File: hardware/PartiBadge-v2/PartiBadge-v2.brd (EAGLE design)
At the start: 119.8 x 118.6 mm, 32 parts, among them J1 I2C, J2 Supply

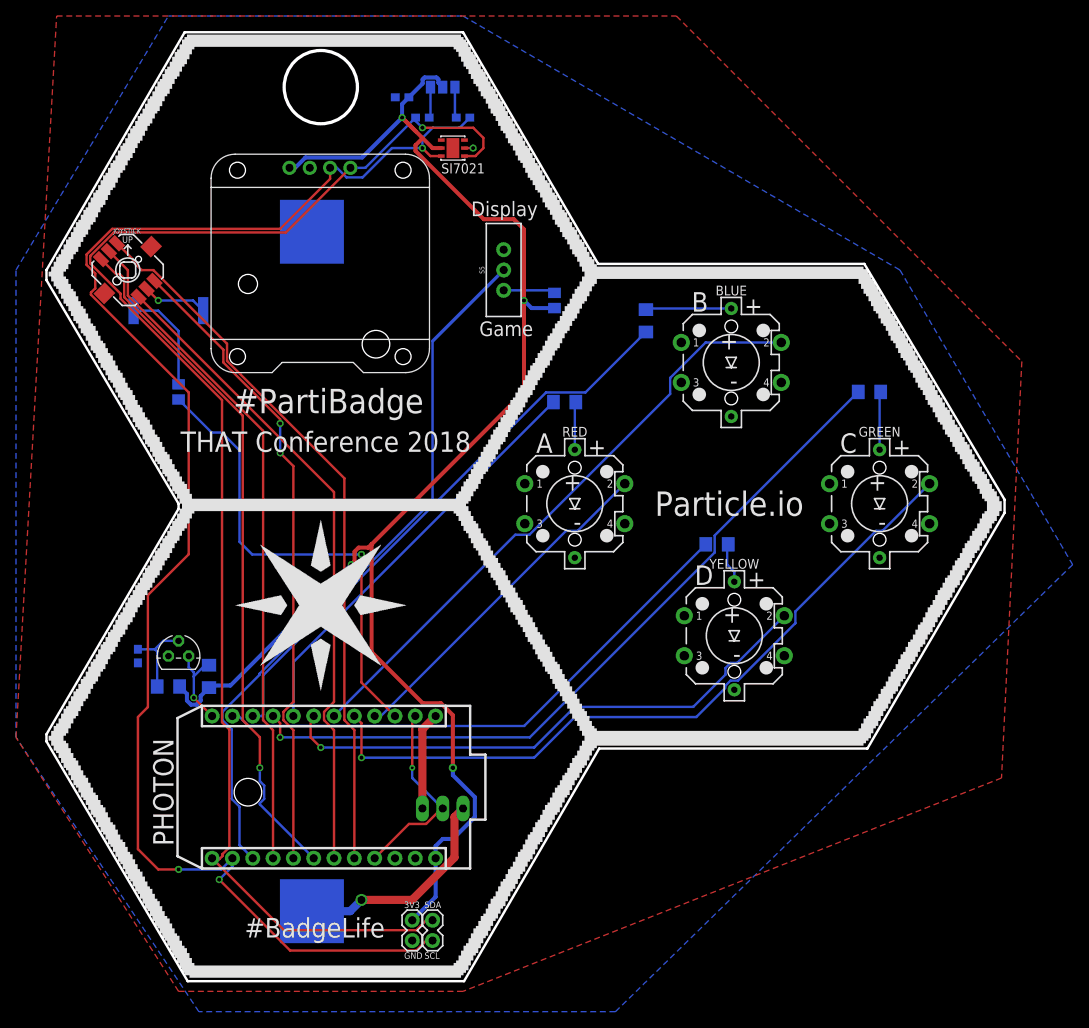
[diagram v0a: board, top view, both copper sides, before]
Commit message: fix v2 board issues
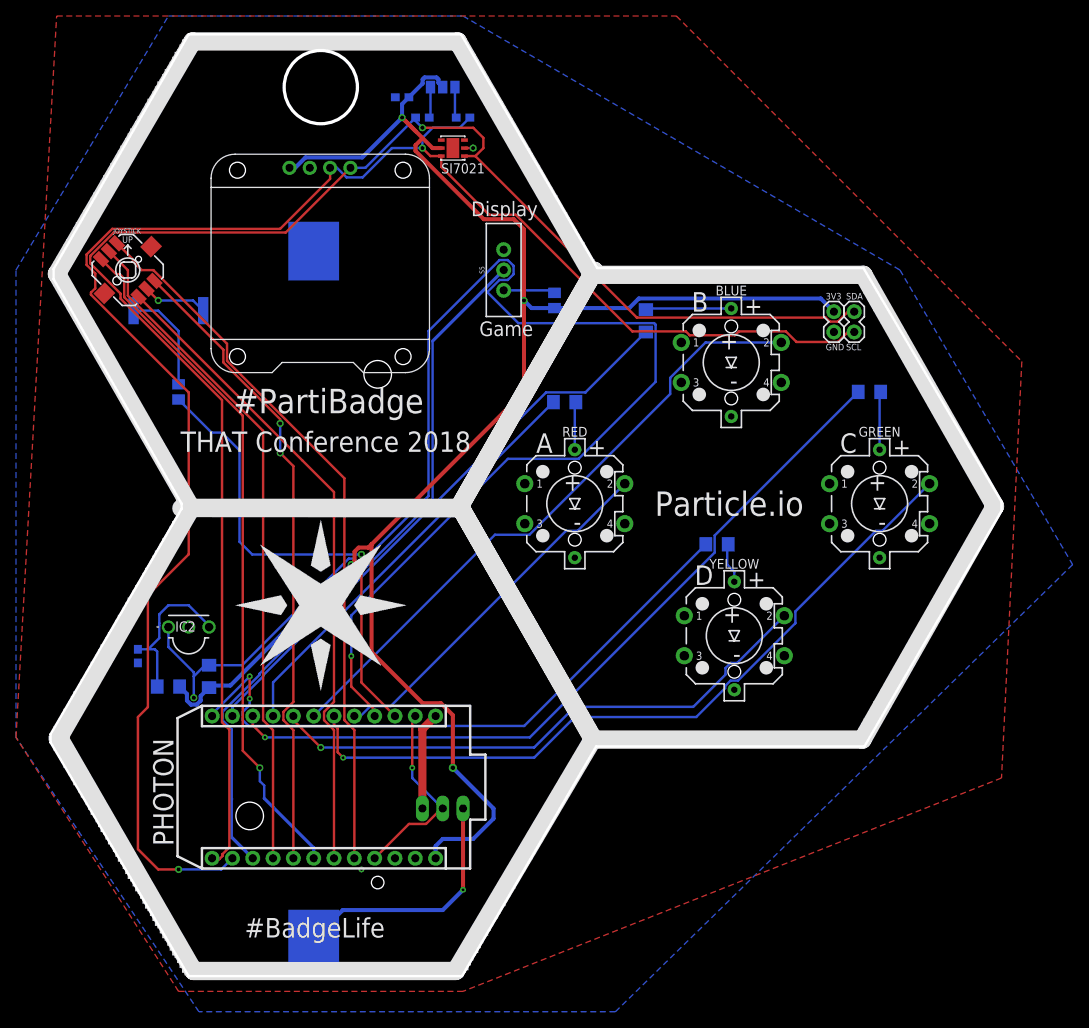
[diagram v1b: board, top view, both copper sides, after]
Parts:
- removed TSMP58000: IR Sensor, transistor-npn:TO92
- removed U$2: SMT18650, SMT18650:18650SMT
- added IC2: TSMP58000, TSMP58000:TSMP58000
- added U1: 1042, 1042:KEYSTONE-1042
- moved J1 92.5 mm to (104.8, 86.2)
- moved J2 92.5 mm to (102.2, 83.7)
- flipped PARTIFRAME to the bottom
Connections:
- removed net VIN: IC1.IN, U$2.BATTERY_POSITIVE
- new net BATT: IC1.IN, U1.2
- net BUTTON_B: now also PHOTON.7; no longer PHOTON.6
- net BUTTON_G: now also PHOTON.6; no longer PHOTON.5
- net BUTTON_R: now also PHOTON.5; no longer PHOTON.4
- net BUTTON_Y: now also PHOTON.8; no longer PHOTON.7
- net GND: now also IC2.2, U1.1; no longer TSMP58000.3, U$2.BATTERY_NEGATIVE
- net IR_RECEIVER: now also IC2.1, PHOTON.4; no longer PHOTON.12, TSMP58000.1
- net LED_B: now also PHOTON.11; no longer PHOTON.10
- net LED_G: now also PHOTON.10; no longer PHOTON.9
- net LED_R: now also PHOTON.9; no longer PHOTON.8
- net LED_Y: now also PHOTON.12; no longer PHOTON.11
- net N$9: now also IC2.3; no longer TSMP58000.2
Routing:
- net IR_RECEIVER: track 11.2 -> 183.7 mm, vias 1 -> 2
- net BATT: track 0.00 -> 31.4 mm, vias 0 -> 1
- net +3V3: track 198.3 -> 228.9 mm
- net SCL: track 190.7 -> 219.4 mm, vias 3 -> 2
- net VIN: track 27.3 -> 0.00 mm, vias 1 -> 0
- net SDA: track 177.5 -> 202.2 mm
- net LED_Y: track 69.1 -> 80.3 mm, vias 0 -> 2
- net N$9: track 10.3 -> 19.8 mm
- net BUTTON_R: track 43.3 -> 45.8 mm
- net BUTTON_B: track 76.4 -> 79.0 mm
- net BUTTON_G: track 91.8 -> 94.2 mm
- net LED_G: track 94.4 -> 96.6 mm
- net LED_R: track 52.7 -> 53.8 mm
- net BUTTON_Y: track 69.9 -> 70.6 mm
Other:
- board size 119.8 x 118.6 mm -> 118.9 x 117.7 mm
